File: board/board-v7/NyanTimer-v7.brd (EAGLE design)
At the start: 136 x 45 mm, 49 parts, among them IC1 7815DT, IC2 MAX232, IC3 7815DT, SW1 AKIZUKI_SWITCH, U1 328P

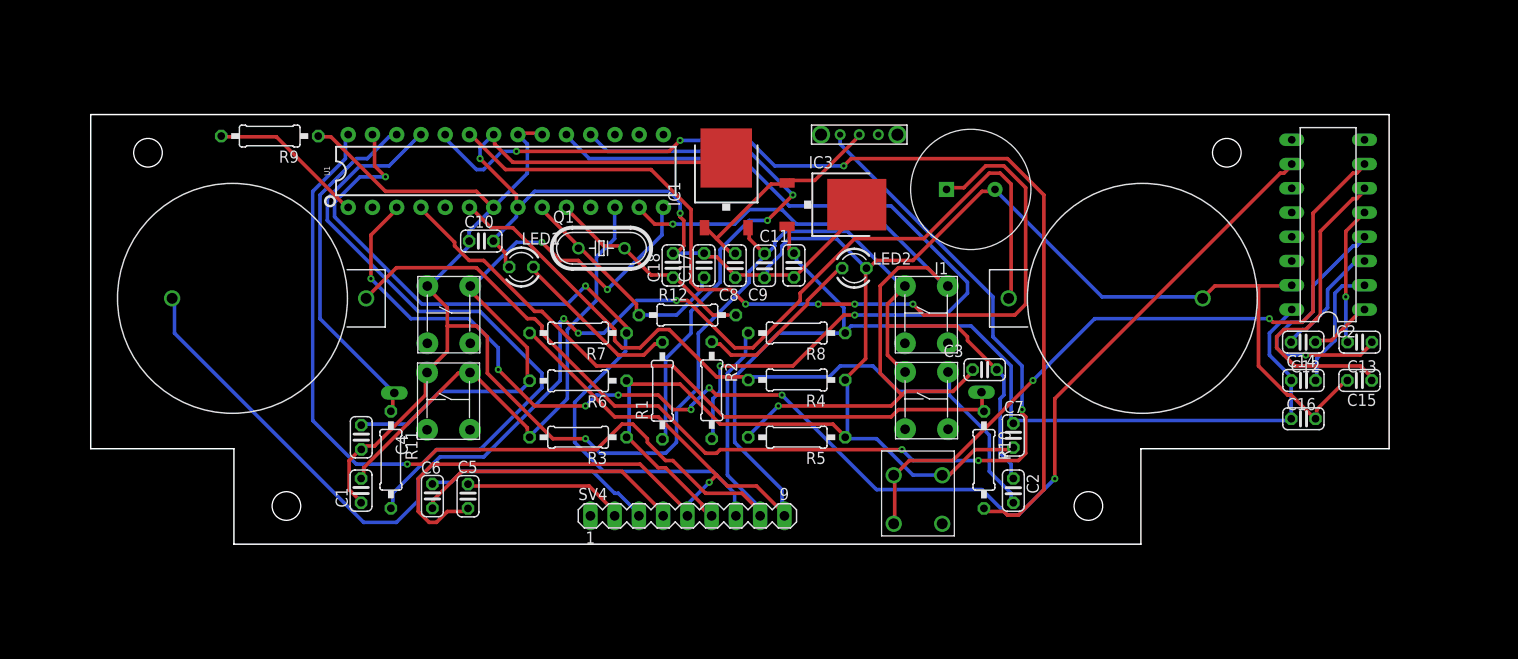
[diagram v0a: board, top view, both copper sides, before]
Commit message: routed
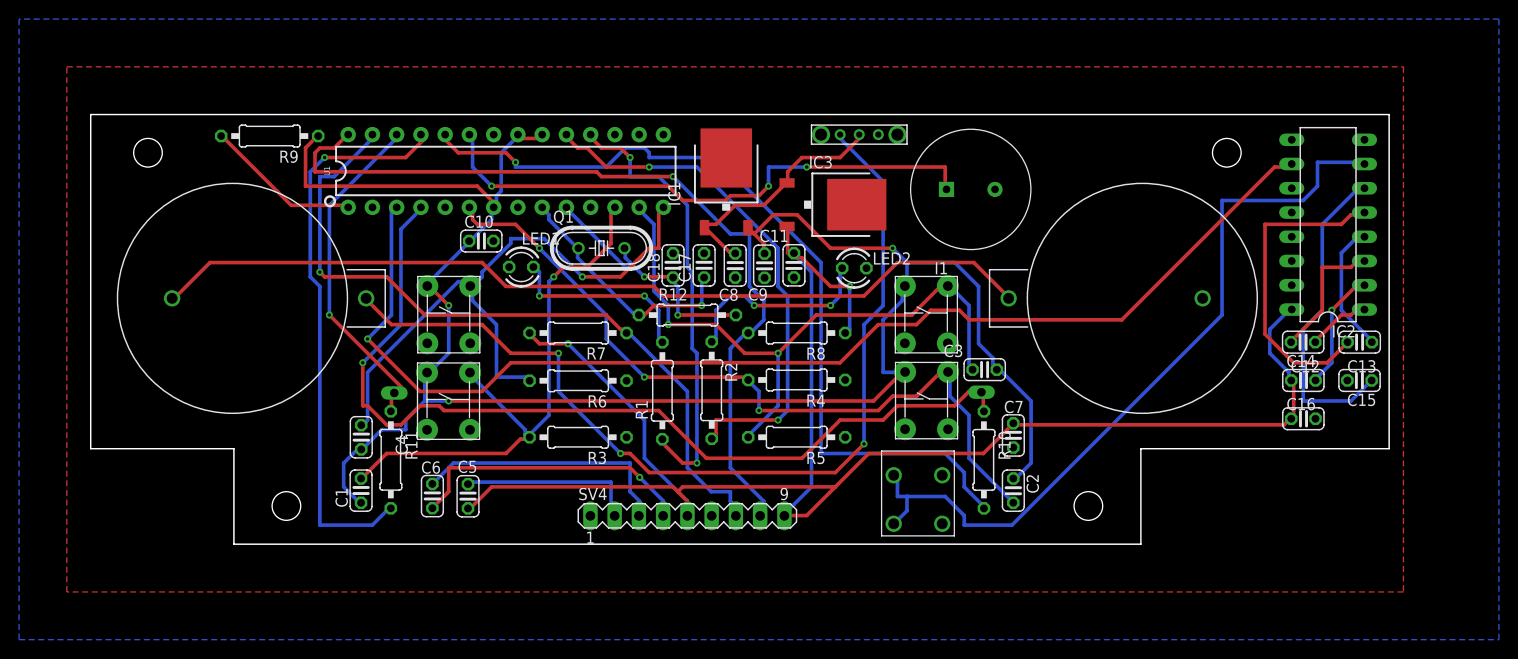
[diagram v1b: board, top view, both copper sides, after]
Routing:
- net GND: track 266.8 -> 0.00 mm, vias 2 -> 0
- net N$7: track 138.1 -> 93.6 mm, vias 3 -> 0
- net BUZ+: track 93.4 -> 59.5 mm, vias 4 -> 3
- net LEDG: track 86.7 -> 54.7 mm
- net PADR: track 70.6 -> 97.0 mm, vias 0 -> 1
- net VSW: track 121.3 -> 98.4 mm
- net SCL: track 108.1 -> 88.2 mm
- net PADRIN: track 107.4 -> 88.0 mm, vias 3 -> 1
- net N$12: track 14.5 -> 33.2 mm, vias 1 -> 0
- net SW3: track 84.7 -> 67.0 mm
- net T2IN: track 139.9 -> 125.2 mm, vias 8 -> 1
- net +5V: track 187.9 -> 201.8 mm, vias 1 -> 3
- net N$11: track 27.2 -> 14.0 mm, vias 1 -> 0
- net LEDR: track 56.3 -> 46.7 mm
- net SDA: track 85.9 -> 77.6 mm, vias 2 -> 1
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- added copper zone on layer 1, net GND
- added copper zone on layer 16, net GND

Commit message: routed
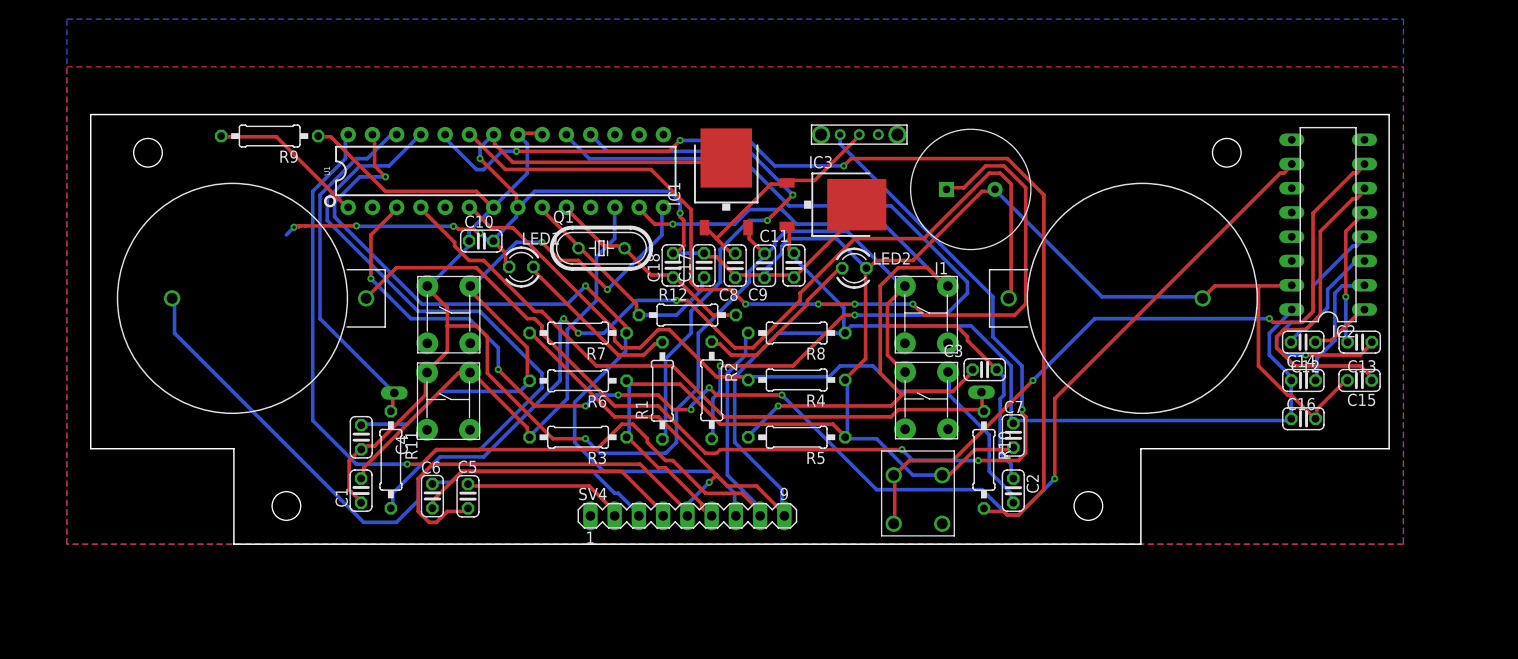
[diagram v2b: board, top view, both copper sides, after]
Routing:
- net GND: track 0.00 -> 289.8 mm, vias 0 -> 6
- net N$7: track 93.6 -> 138.1 mm, vias 0 -> 3
- net BUZ+: track 59.5 -> 93.4 mm, vias 3 -> 4
- net LEDG: track 54.7 -> 86.7 mm
- net PADR: track 97.0 -> 70.6 mm, vias 1 -> 0
- net VSW: track 98.4 -> 121.3 mm
- net SCL: track 88.2 -> 108.1 mm
- net PADRIN: track 88.0 -> 107.4 mm, vias 1 -> 3
- net N$12: track 33.2 -> 14.5 mm, vias 0 -> 1
- net SW3: track 67.0 -> 84.7 mm
- net T2IN: track 125.2 -> 139.9 mm, vias 1 -> 8
- net +5V: track 201.8 -> 187.9 mm, vias 3 -> 1
- net N$11: track 14.0 -> 27.2 mm, vias 0 -> 1
- net LEDR: track 46.7 -> 56.3 mm
- net SDA: track 77.6 -> 85.9 mm, vias 1 -> 2
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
